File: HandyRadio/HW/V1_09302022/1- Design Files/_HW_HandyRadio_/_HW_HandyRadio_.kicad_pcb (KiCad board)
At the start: 4 copper layers, 74.9 x 74.9 mm, 173 parts, among them J301 MHDR_4POS_1ROW, J302 RECEP_6POS_1ROW, J401 XH_CONN_2POS_R/A, J501 USB_uAB_RECEP, J502 XH_CONN_2POS_R/A, J801 MHDR_2POS_VERT, K801 DPDT_RELAY, Q501 IRF7401TRPBF, Q801 MMUN2215LT1G, SW301 SPST_NO_RA, SW302 SPST_NO_RA, SW303 SPST_NO_RA, U301 PIC16F15223, U302 IR_REC_38KHz, U401 PAM8302AASCR, U501 MCP73831, U502 AP7361EA, U503 R1211N002B, U504 MIC5365-3.3, U801 EGUARD0502A, U802 SI4735-D60-GU

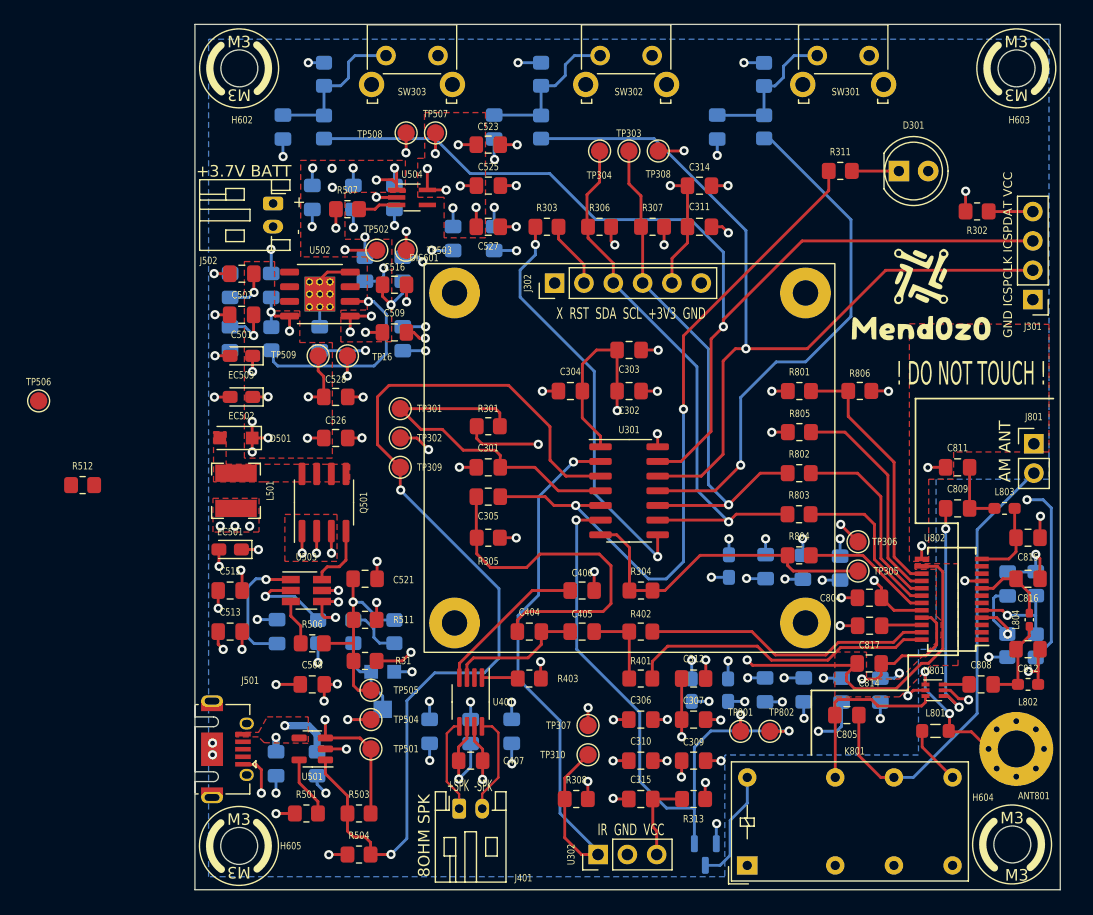
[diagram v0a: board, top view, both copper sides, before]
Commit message: Serious changes in placement
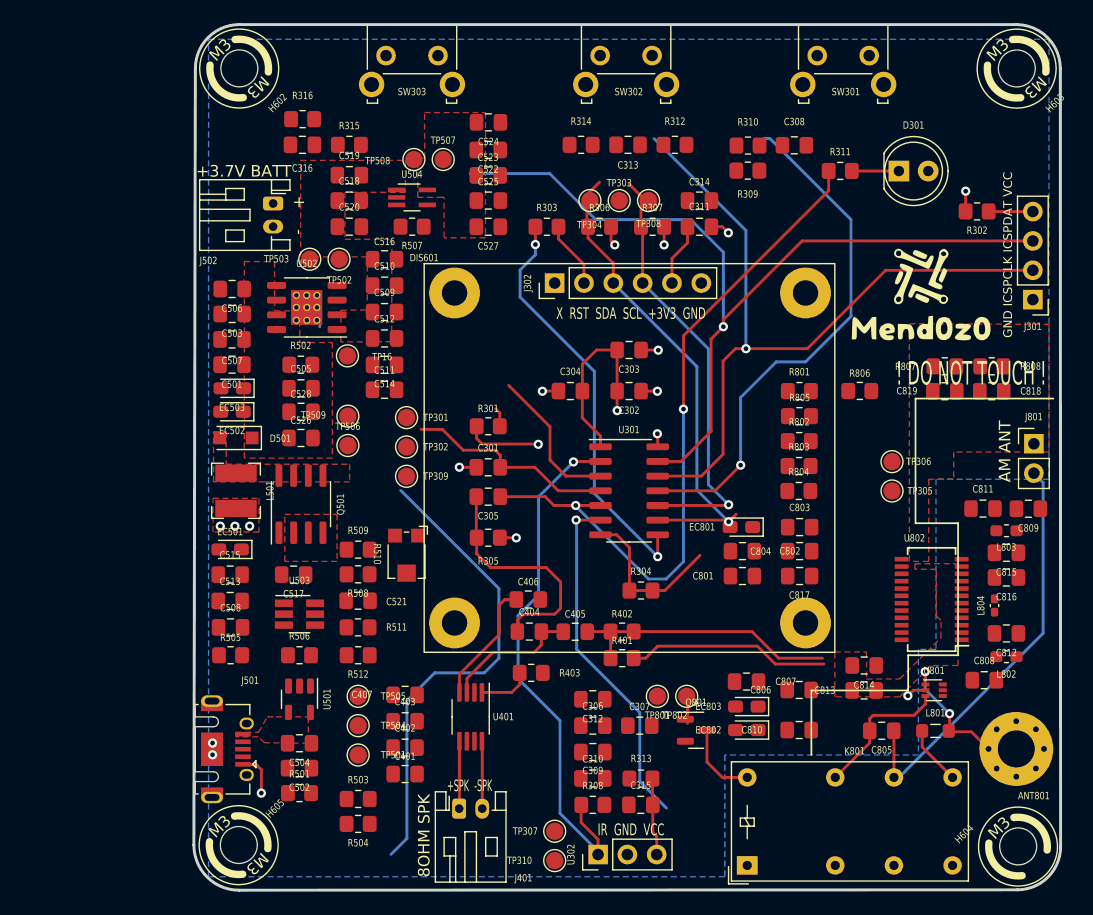
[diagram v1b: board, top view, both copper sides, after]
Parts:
- removed R31: 16KR5, Resistor_SMD:R_0805_2012Metric_Pad1.20x1.40mm_HandSolder
- C308, C313, C316, C401, C402, C403, C502, C503, C504, C505, C506, C510, C511, C512, C514, C517, C518, C519, C520, C522, C524, C801, C802, C803, C806, C807, C810, C813, C818, C819, EC801, EC802, EC803, Q801, R309, R310, R312, R314, R315, R316, R502, R505, R508, R509, R510, R807, R808: moved to F.Cu
- moved R512 28.0 mm to (197.0, 160.0), turned to 180 degrees
- moved TP506 27.1 mm to (196.1, 141.9)
- moved R807 25.5 mm to (247.8, 135.0), turned to 180 degrees
- moved R808 24.2 mm to (251.9, 135.0), turned to 0 degrees
- moved C819 18.4 mm to (247.8, 137.2), turned to 0 degrees
- moved C818 16.7 mm to (251.9, 137.2), turned to 180 degrees
- moved R510 12.3 mm to (201.9, 148.8)
- moved C313 11.7 mm to (220.4, 115.8), turned to 0 degrees
- moved R312 11.7 mm to (224.4, 115.8), turned to 180 degrees
- moved C807 11.6 mm to (230.6, 162.3), turned to 0 degrees
- moved Q801 10.8 mm to (226.3, 166.5), turned to 0 degrees
- moved C524 10.1 mm to (208.3, 113.9), turned to 180 degrees
- moved TP307 9.60 mm to (214.0, 175.3)
- moved TP310 9.60 mm to (214.0, 177.8)
- moved C403 9.28 mm to (201.1, 165.8), turned to 0 degrees
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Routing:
- net GND: track 202.2 -> 17.7 mm, vias 96 -> 11
- net +5V: track 65.5 -> 0.00 mm, vias 26 -> 0
- net +3V3: track 97.8 -> 33.6 mm, vias 30 -> 5
- net /BLOCK DIAGRAM/MCU, RTC, OLED, PB, LED/BATT_STAT: track 87.2 -> 54.3 mm, vias 2 -> 0
- net +6V: track 30.0 -> 0.00 mm, vias 13 -> 0
- net +BATT: track 24.5 -> 0.00 mm, vias 12 -> 3
- net /BLOCK DIAGRAM/RF RECEIVER/~{RST}: track 22.2 -> 0.00 mm
- net Net-(C809-Pad1): track 19.5 -> 0.00 mm, vias 2 -> 0
- net /BLOCK DIAGRAM/RF RECEIVER/~{SEN}: track 19.1 -> 0.00 mm
- net /BLOCK DIAGRAM/MCU, RTC, OLED, PB, LED/~{FM}/SW_SEL: track 51.5 -> 32.7 mm, vias 2 -> 1
- net Net-(R502-Pad2): track 18.5 -> 0.00 mm, vias 1 -> 0
- net Net-(C521-Pad1): track 17.7 -> 0.00 mm, vias 1 -> 0
- net /BLOCK DIAGRAM/RF RECEIVER/SCLK: track 16.9 -> 0.00 mm
- net /BLOCK DIAGRAM/MCU, RTC, OLED, PB, LED/SI47_CLK: track 28.8 -> 14.1 mm
- net /BLOCK DIAGRAM/RF RECEIVER/SDIO: track 14.3 -> 0.00 mm
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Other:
- board size 74.9 x 74.9 mm -> 75 x 75 mm
- board text removed: "M3"
